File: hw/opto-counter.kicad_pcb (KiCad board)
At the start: 2 copper layers, 27.9 x 27.9 mm, 13 parts, among them J1 IR-REC, J2 qwiic, J3 UPDI, U1 ATtiny3224-SS, U2 TSSP6038

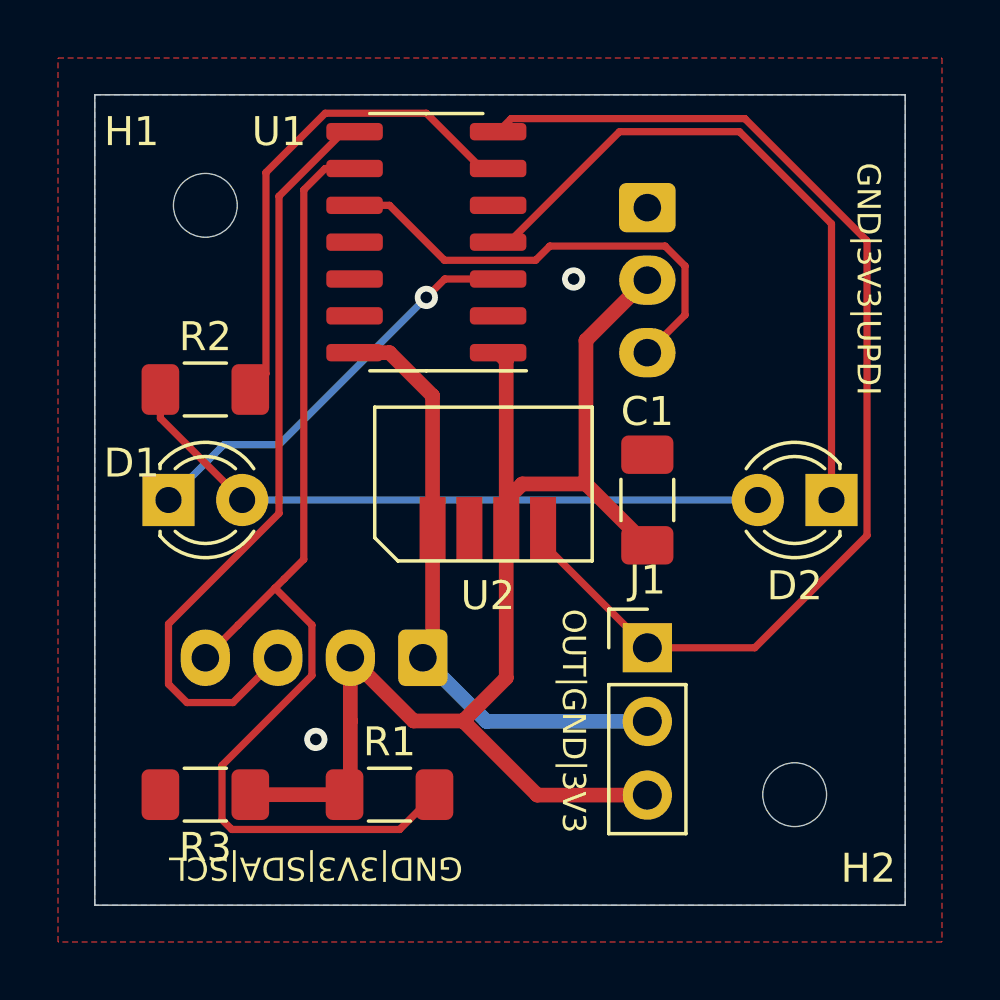
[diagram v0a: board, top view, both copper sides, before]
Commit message: Some more work on fixing the PCB
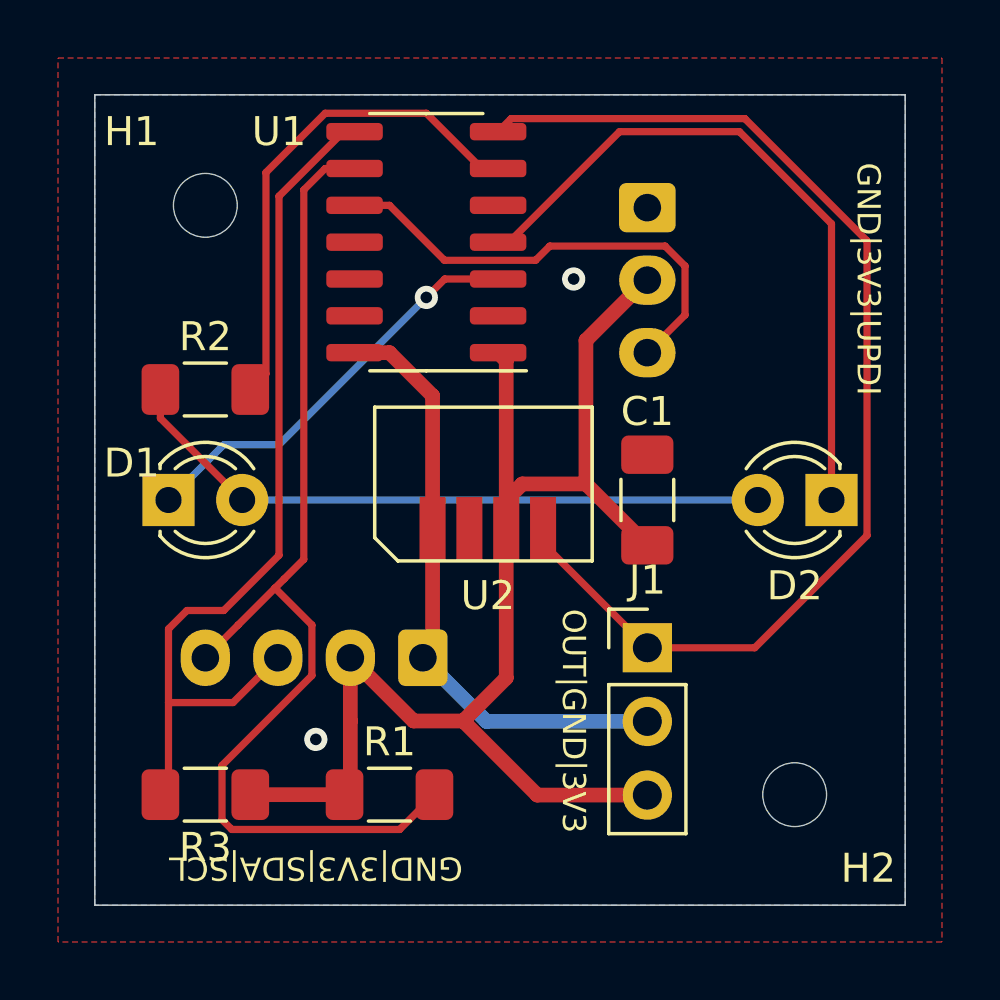
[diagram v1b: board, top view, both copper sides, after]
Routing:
- net SDA: track 26.6 -> 31.0 mm
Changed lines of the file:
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@@
   (segment (start 88.9 28.575) (end 88.9 38.1) (width 0.25) (layer "F.Cu") (net 5))
   (segment (start 81.591751 25.4) (end 85.725 25.4) (width 0.25) (layer "F.Cu") (net 5))
-  (segment (start 66.675 45.085) (end 68.265 45.085) (width 0.25) (layer "F.Cu") (net 6))
-  (segment (start 66.04 42.372412) (end 69.85 38.562412) (width 0.25) (layer "F.Cu") (net 6))
-  (segment (start 72.075457 25.4) (end 72.455 25.4) (width 0.25) (layer "F.Cu") (net 6))
-  (segment (start 69.85 38.562412) (end 69.85 27.625457) (width 0.25) (layer "F.Cu") (net 6))
-  (segment (start 69.85 27.625457) (end 72.075457 25.4) (width 0.25) (layer "F.Cu") (net 6))
-  (segment (start 66.04 44.45) (end 66.675 45.085) (width 0.25) (layer "F.Cu") (net 6))
-  (segment (start 66.04 42.372412) (end 66.04 44.45) (width 0.25) (layer "F.Cu") (net 6))
-  (segment (start 68.265 45.085) (end 69.81 43.54) (width 0.25) (layer "F.Cu") (net 6))
+  (segment (start 66.04 47.98) (end 66.04 45.085) (width 0.25) (layer "F.Cu") (net 6))
+  (segment (start 68.265 45.085) (end 66.04 45.085) (width 0.25) (layer "F.Cu") (net 6))
+  (segment (start 72.075457 25.4) (end 69.85 27.625457) (width 0.25) (layer "F.Cu") (net 6))
+  (segment (start 67.945 41.91) (end 66.675 41.91) (width 0.25) (layer "F.Cu") (net 6))
+  (segment (start 65.76 48.26) (end 66.04 47.98) (width 0.25) (layer "F.Cu") (net 6))
+  (segment (start 69.81 43.54) (end 68.265 45.085) (width 0.25) (layer "F.Cu") (net 6))
+  (segment (start 66.675 41.91) (end 66.04 42.545) (width 0.25) (layer "F.Cu") (net 6))
+  (segment (start 69.85 40.005) (end 67.945 41.91) (width 0.25) (layer "F.Cu") (net 6))
+  (segment (start 69.85 27.625457) (end 69.85 40.005) (width 0.25) (layer "F.Cu") (net 6))
+  (segment (start 66.04 42.545) (end 66.04 45.085) (width 0.25) (layer "F.Cu") (net 6))
+  (segment (start 72.455 25.4) (end 72.075457 25.4) (width 0.25) (layer "F.Cu") (net 6))
   (segment (start 70.03 40.82) (end 69.7125 41.1375) (width 0.25) (layer "F.Cu") (net 7))
   (segment (start 74.01 49.46) (end 68.221827 49.46) (width 0.25) (layer "F.Cu") (net 7))
